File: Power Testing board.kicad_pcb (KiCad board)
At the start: 2 copper layers, 170 x 130 mm, 96 parts, among them J1 J_ATX_PWR: 3V3 3V3 5V 5V 12V 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, J2 J_ATX_CTRL: PS_ON PWR_OK 5VSB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, J3 ATX_SWITCH, J4 DEDICATED OUTPUTS: 3V3/G 5V/G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, Q1 2N7002 RESET_3V3 pulldown, Q2 2N7002 RESET_5V pulldown, Q3 2N7002 RESET_12V pulldown, Q4 2N7002 RESET_16V8 pulldown, Q5 2N7002 ATX PS_ON# pulldown, SW1 RESET_3V3 edge button, SW2 RESET_5V edge button, SW3 RESET_12V edge button, SW4 RESET_16V8 edge button, U1 TPS259814L 3V3 eFuse latch-off, U2 TPS26631RGE 5V eFuse, U3 TPS26631RGE 12V eFuse, U4 TPS26631RGE 16V8 eFuse, U5 INA260 3V3 module, U6 INA260 5V module, U7 INA260 12V module, U8 INA260 16V8 module, U9 Boost 12V to 16.8V module 60x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

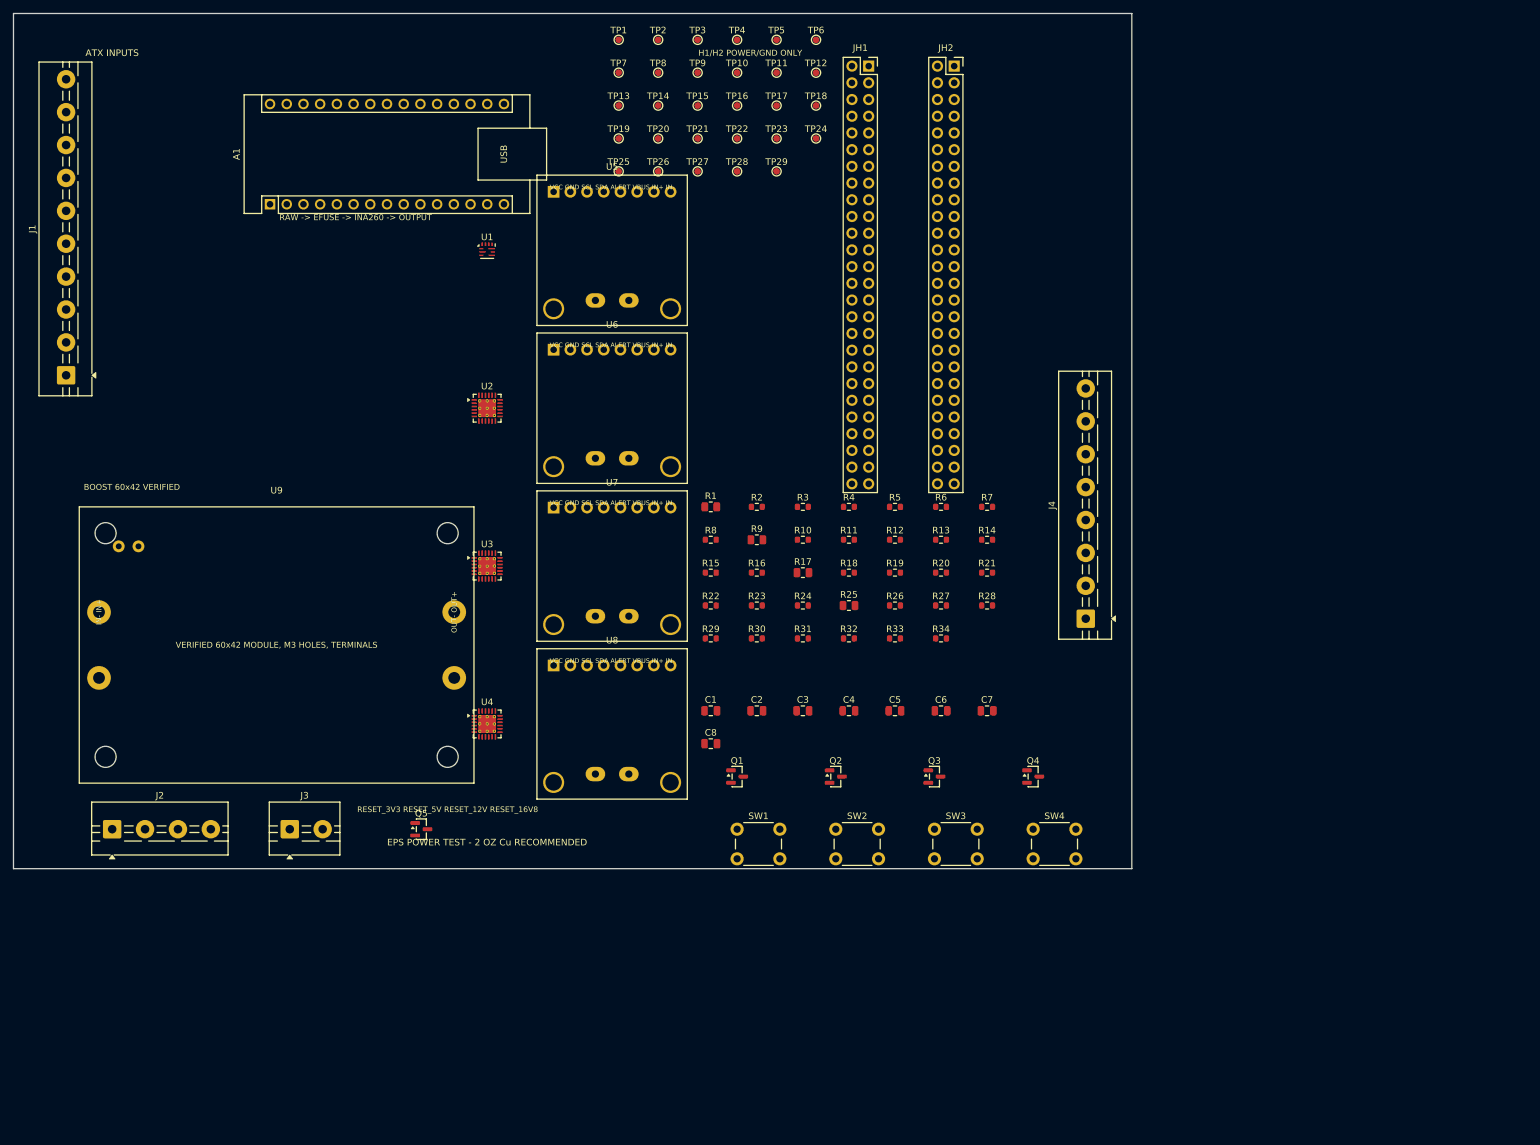
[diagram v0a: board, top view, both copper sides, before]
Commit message: chat gpt pt.2
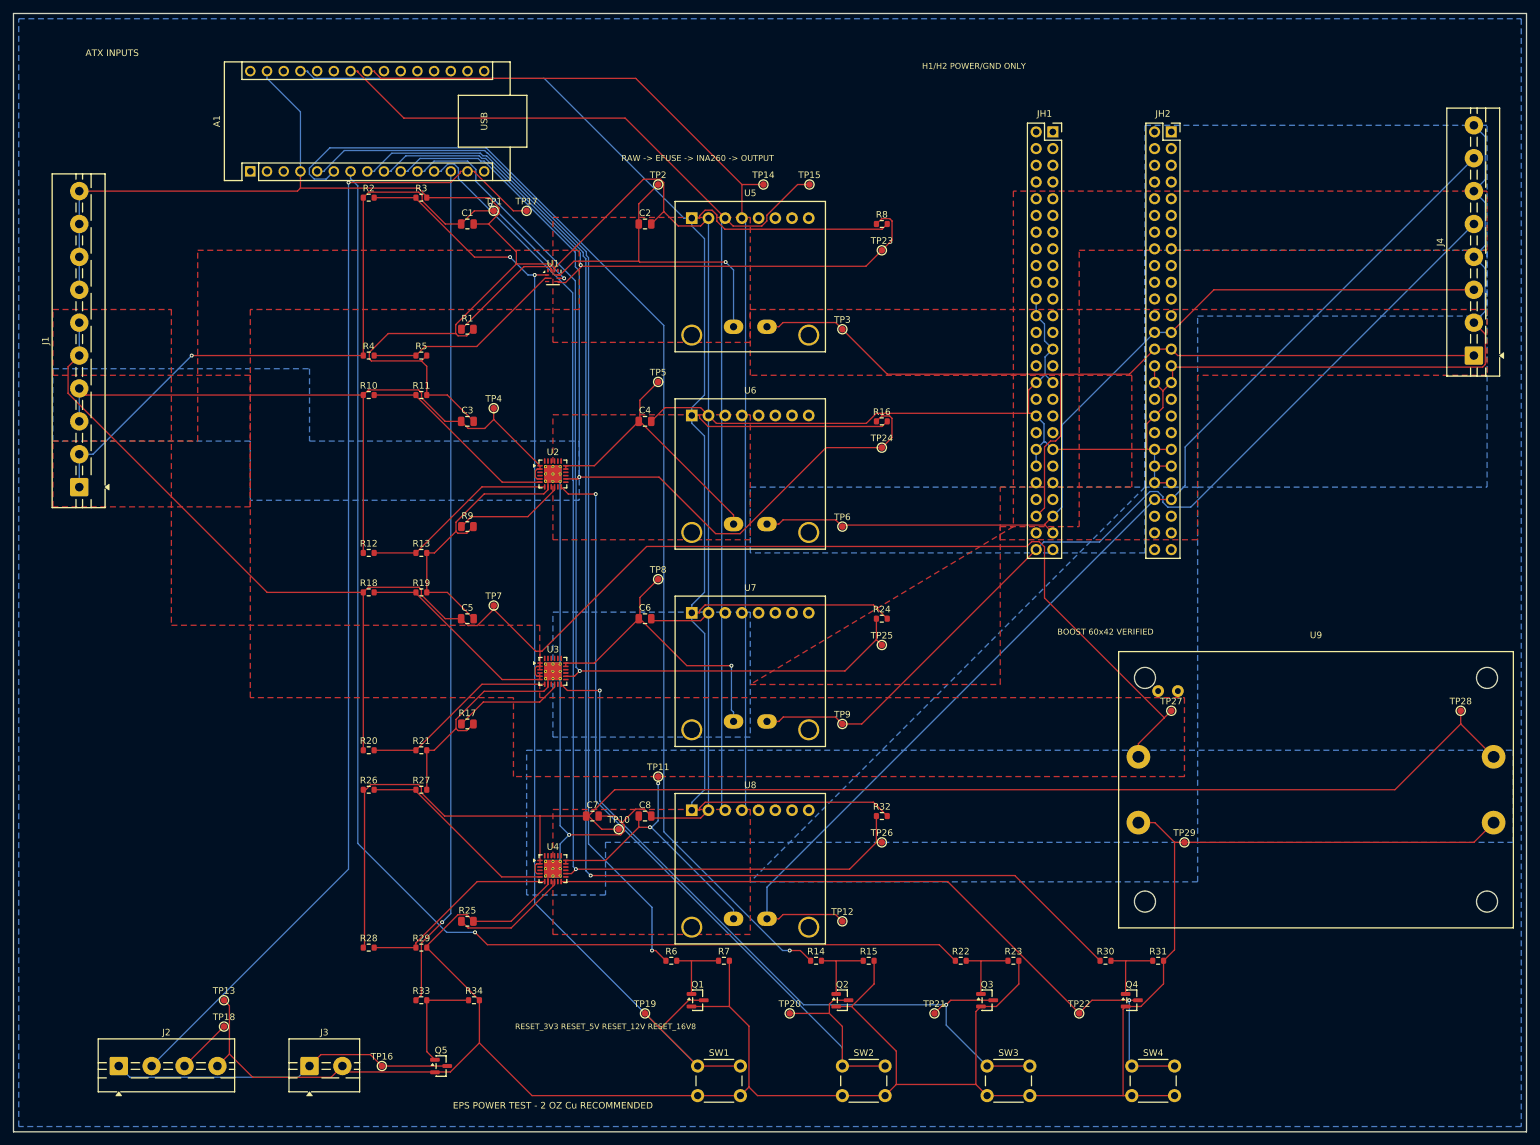
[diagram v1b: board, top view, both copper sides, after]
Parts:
- C1, C3: value 1uF input close to eFuse -> 1uF 25V X7R input close to eFuse
- C2, C4: value 10uF output close to eFuse -> 10uF 25V X7R output close to eFuse
- C5, C7: value 1uF input close to eFuse -> 1uF 50V X7R input close to eFuse
- C6, C8: value 10uF output close to eFuse -> 10uF 50V X7R output close to eFuse
- R10: value 249k UVLO top -> 261k 1% UVLO top 4.33V
- R11, R19, R27: value 100k UVLO bottom -> 100k 1% UVLO bottom
- R12: value 402k OVP top -> 383k 1% OVP top 5.80V
- R13, R21, R29: value 100k OVP bottom -> 100k 1% OVP bottom
- R18: value 649k UVLO top -> 806k 1% UVLO top 10.87V
- R2: value 100k EN top -> 100k 1% EN top 2.40V
- R20: value 1.15M OVP top -> 1.05M 1% OVP top 13.80V
- R26: value 976k UVLO top -> 1.07M 1% UVLO top 14.04V
- R28: value 1.50M OVP top -> 1.40M 1% OVP top 18.00V
- R3: value 100k EN bottom -> 100k 1% EN bottom
- R4: value 24.9k OVLO top -> 24.9k 1% OVLO top 4.19V
- R5: value 10k OVLO bottom -> 10k 1% OVLO bottom
- moved TP18 166.4 mm to (32.0, 154.0)
- moved U9 159.5 mm to (198.0, 118.0)
- moved TP16 155.7 mm to (56.0, 160.0)
- moved TP13 148.6 mm to (32.0, 150.0)
- moved TP22 142.8 mm to (162.0, 152.0)
- moved TP21 137.8 mm to (140.0, 152.0)
- moved TP28 137.2 mm to (220.0, 106.0)
- moved TP20 134.5 mm to (118.0, 152.0)
- moved TP19 133.1 mm to (96.0, 152.0)
- moved TP12 129.1 mm to (126.0, 138.0)
- moved TP29 119.4 mm to (178.0, 126.0)
- moved TP10 116.4 mm to (92.0, 124.0)
- moved TP27 109.1 mm to (176.0, 106.0)
- moved TP11 108.5 mm to (98.0, 116.0)
- moved TP26 107.5 mm to (132.0, 126.0)
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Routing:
- net GND: track 0.00 -> 1112.5 mm, vias 0 -> 1
- net +ARDUINO_5V: track 0.00 -> 289.7 mm
- net +12V_RAW: track 0.00 -> 258.6 mm
- net +16V8_RAW: track 0.00 -> 223.9 mm
- net ARD_RESET_16V8: track 0.00 -> 218.3 mm, vias 0 -> 1
- net ARD_RESET_12V: track 0.00 -> 200.8 mm, vias 0 -> 1
- net RESET_3V3: track 0.00 -> 188.0 mm, vias 0 -> 2
- net ARD_RESET_5V: track 0.00 -> 179.2 mm, vias 0 -> 1
- net ATX_PWR_OK: track 0.00 -> 177.2 mm, vias 0 -> 1
- net I2C_SCL: track 0.00 -> 174.1 mm
- net +16V8_PROTECTED: track 0.00 -> 173.8 mm
- net FLT_16V8: track 0.00 -> 172.5 mm, vias 0 -> 1
- net I2C_SDA: track 0.00 -> 163.9 mm
- net ARD_RESET_3V3: track 0.00 -> 161.8 mm, vias 0 -> 1
- net FLT_12V: track 0.00 -> 146.8 mm, vias 0 -> 1
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- added copper zone on B.Cu, net +12V_EFUSE_OUT
- added copper zone on F.Cu, net +12V_PROTECTED
- added copper zone on F.Cu, net +12V_RAW
- added copper zone on F.Cu, net +16V8_EFUSE_OUT
- added copper zone on B.Cu, net +16V8_PROTECTED
- added copper zone on B.Cu, net +16V8_RAW
- added copper zone on F.Cu, net +3V3_EFUSE_OUT
- added copper zone on F.Cu, net +3V3_PROTECTED
- added copper zone on F.Cu, net +3V3_RAW
- added copper zone on F.Cu, net +5V_EFUSE_OUT
- added copper zone on B.Cu, net +5V_PROTECTED
- added copper zone on B.Cu, net +5V_RAW
- added copper zone on B.Cu, net GND
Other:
- board size 170 x 130 mm -> 230 x 170 mm
